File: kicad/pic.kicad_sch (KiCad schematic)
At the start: 2 parts, among them U60 8259

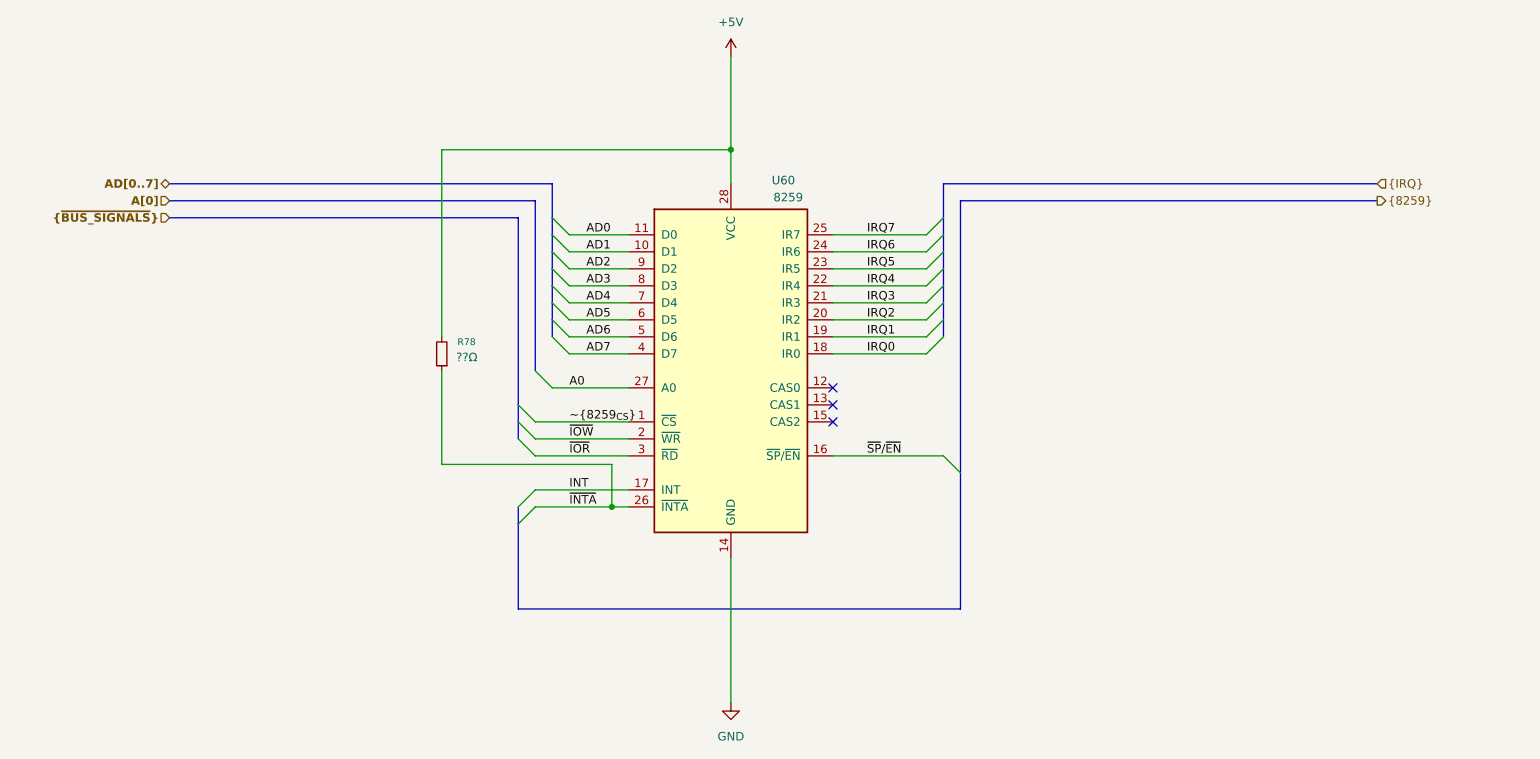
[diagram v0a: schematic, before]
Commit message: update kicad project
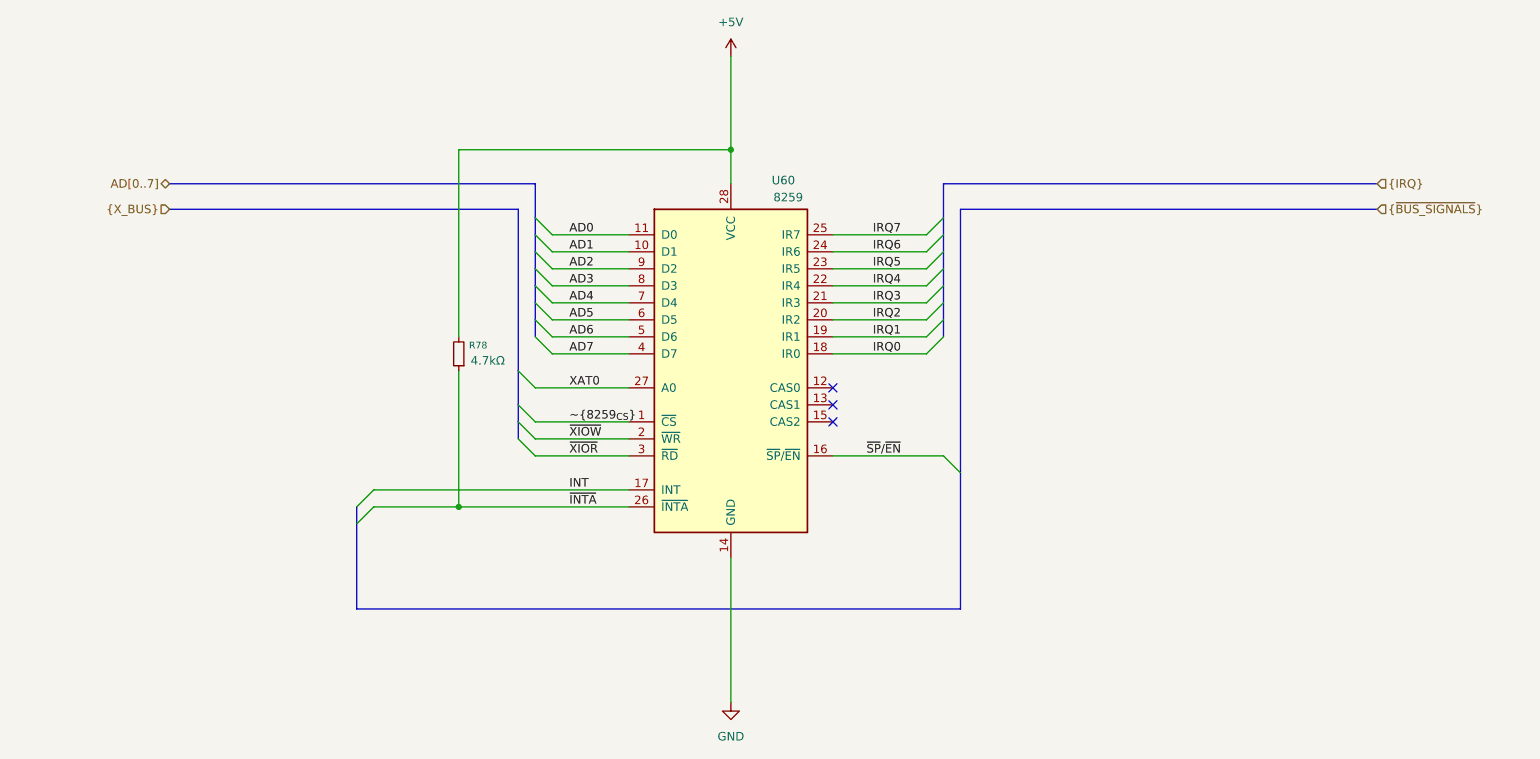
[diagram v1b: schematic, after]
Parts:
- R78: value ??Ω -> 4.7kΩ; seq_coord (none) -> E15; seq_notes (none) -> Yellow,Violet,Red,Gold
- U60: seq_coord (none) -> D14; seq_silkscreen (none) -> 8259
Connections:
- net A0 renamed XAT0
- net ~{IOR} renamed ~{XIOR}
- net ~{IOW} renamed ~{XIOW}
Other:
- moved on the sheet: R78
